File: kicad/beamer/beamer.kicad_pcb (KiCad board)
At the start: 2 copper layers, 117.3 x 83 mm, 65 parts

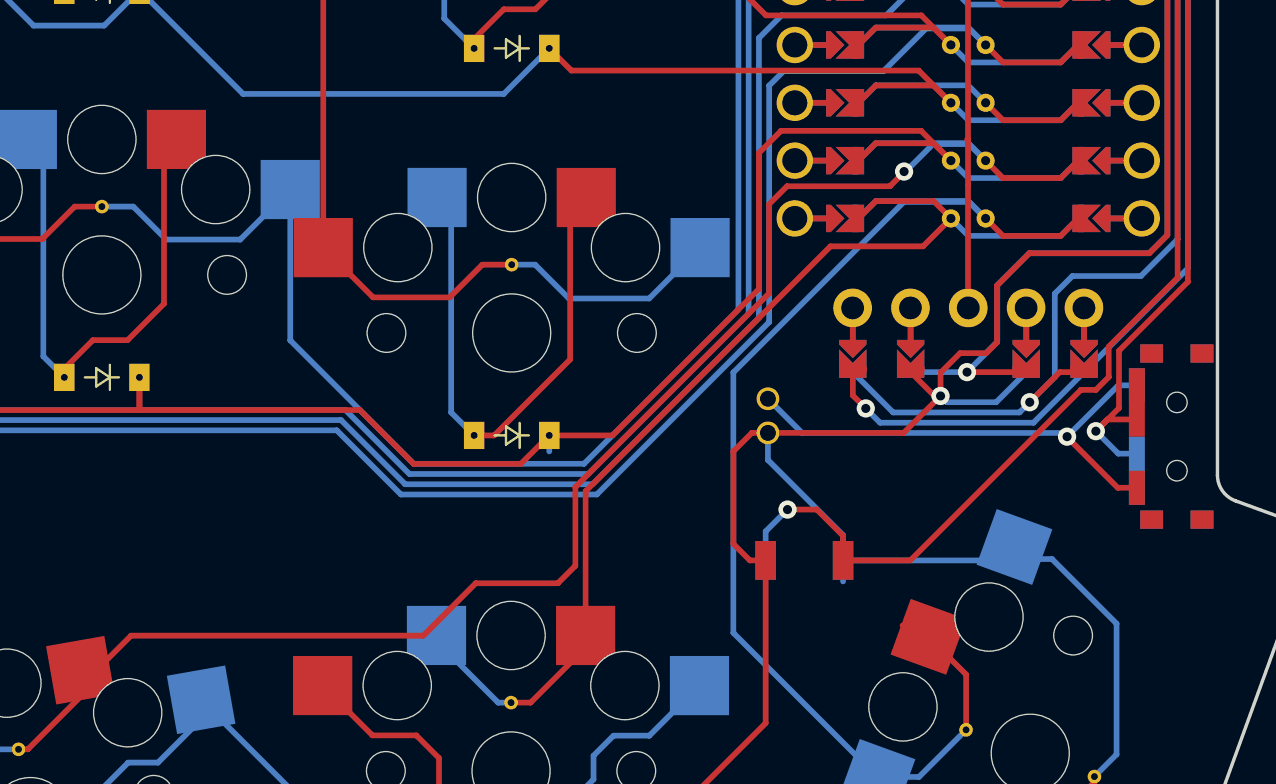
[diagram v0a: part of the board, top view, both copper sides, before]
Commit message: Final changes for printing
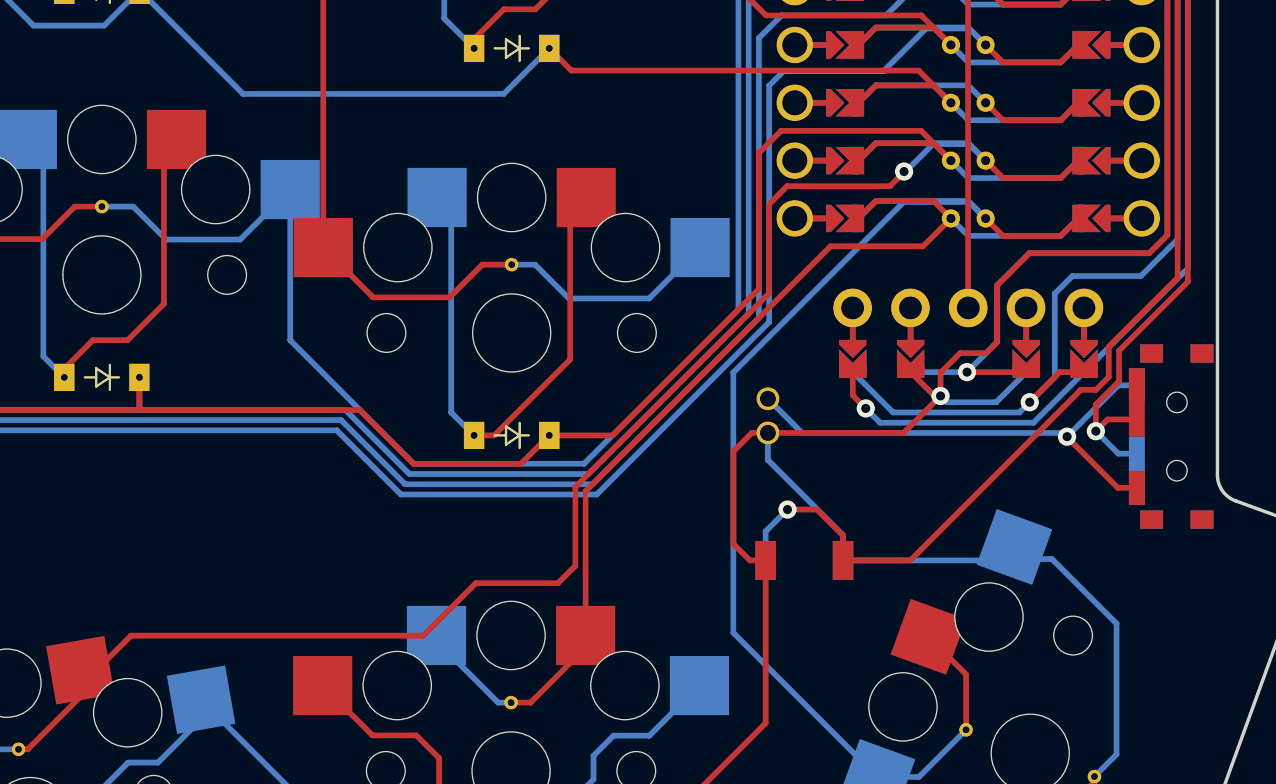
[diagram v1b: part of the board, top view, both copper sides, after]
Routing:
- net P10: track 45.6 -> 44.4 mm
- net GND: track 200.3 -> 199.4 mm
- net P8: track 117.0 -> 116.1 mm
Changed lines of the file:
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@@
       (outputformat 1)
       (mirror false)
-      (drillshape 1)
+      (drillshape 0)
       (scaleselection 1)
-      (outputdirectory "")
+      (outputdirectory "Gerber/")
     )
   )
@@
   (segment (start 158.65 161.2) (end 160.700382 161.2) (width 0.25) (layer "F.Cu") (net 3))
   (segment (start 176.65 149.259378) (end 176.65 148.45) (width 0.25) (layer "F.Cu") (net 3))
-  (segment (start 212.65 148.45) (end 212.65 148.6) (width 0.25) (layer "F.Cu") (net 3))
   (segment (start 222.32912 149.886002) (end 224.693899 152.250781) (width 0.25) (layer "F.Cu") (net 3))
   (segment (start 175.901789 150.007589) (end 176.65 149.259378) (width 0.25) (layer "F.Cu") (net 3))
@@
   (segment (start 239.86 138.594959) (end 240.834601 137.620358) (width 0.25) (layer "F.Cu") (net 3))
   (segment (start 180.054638 148.45) (end 182.292485 146.212153) (width 0.25) (layer "F.Cu") (net 3))
-  (segment (start 230.65 151.704121) (end 230.65 151) (width 0.25) (layer "B.Cu") (net 3))
   (segment (start 159.670356 134.354644) (end 159.670356 140.855062) (width 0.25) (layer "F.Cu") (net 4))
   (segment (start 159.670356 140.855062) (end 157.960229 142.565189) (width 0.25) (layer "F.Cu") (net 4))
@@
   (segment (start 235.045994 164.189093) (end 233.472621 164.189093) (width 0.25) (layer "B.Cu") (net 25))
   (segment (start 243.555 156.49) (end 250.493904 156.49) (width 0.25) (layer "B.Cu") (net 25))
-  (segment (start 243.555 156.49) (end 243.555 157.414572) (width 0.25) (layer "B.Cu") (net 25))
   (segment (start 229.967611 168.737433) (end 228.972654 168.737433) (width 0.25) (layer "B.Cu") (net 25))
   (segment (start 232.594895 165.066819) (end 232.594895 166.110149) (width 0.25) (layer "B.Cu") (net 25))
@@
   (segment (start 251.613064 156.429604) (end 252.731637 156.429604) (width 0.25) (layer "B.Cu") (net 25))
   (segment (start 248.111903 149.541729) (end 250.281271 149.541729) (width 0.25) (layer "B.Cu") (net 25))
-  (segment (start 246.169237 159.345616) (end 246.98806 160.164439) (width 0.25) (layer "F.Cu") (net 26))
   (segment (start 247.306258 159.846241) (end 248.958235 161.498218) (width 0.25) (layer "F.Cu") (net 26))
   (segment (start 248.958235 161.498218) (end 248.958235 163.932694) (width 0.25) (layer "F.Cu") (net 26))
@@
   (segment (start 228.407591 162.737433) (end 228.972654 162.737433) (width 0.25) (layer "B.Cu") (net 27))
   (segment (start 225.697654 159.787433) (end 225.697654 160.027496) (width 0.25) (layer "B.Cu") (net 27))
-  (segment (start 257.254622 114.799263) (end 251.086263 114.799263) (width 0.25) (layer "F.Cu") (net 28))
   (segment (start 254.659212 150.814567) (end 255.173779 150.3) (width 0.25) (layer "F.Cu") (net 28))
-  (segment (start 258.7 116.244641) (end 257.254622 114.799263) (width 0.25) (layer "F.Cu") (net 28))
+  (segment (start 258.7 144.26) (end 258.7 116.244641) (width 0.25) (layer "F.Cu") (net 28))
   (segment (start 255.173779 150.3) (end 256.46 150.3) (width 0.25) (layer "F.Cu") (net 28))
-  (segment (start 256.46 150.3) (end 256.177 150.3) (width 0.25) (layer "F.Cu") (net 28))
-  (segment (start 254.659212 150.814567) (end 255.675947 149.797832) (width 0.25) (layer "F.Cu") (net 28))
-  (segment (start 251.086263 114.799263) (end 249.817 113.53) (width 0.25) (layer "F.Cu") (net 28))
-  (segment (start 255.675947 149.797832) (end 255.675947 147.284053) (width 0.25) (layer "F.Cu") (net 28))
   (segment (start 255.675947 147.284053) (end 258.7 144.26) (width 0.25) (layer "F.Cu") (net 28))
-  (segment (start 258.7 144.26) (end 258.7 116.244641) (width 0.25) (layer "F.Cu") (net 28))
+  (segment (start 257.254622 114.799263) (end 251.086263 114.799263) (width 0.25) (layer "F.Cu") (net 28))
+  (segment (start 254.659212 150.814567) (end 254.659212 149.640184) (width 0.25) (layer "F.Cu") (net 28))
+  (segment (start 254.659212 149.640184) (end 255.675947 148.623449) (width 0.25) (layer "F.Cu") (net 28))
+  (segment (start 251.086263 114.799263) (end 249.817 113.53) (width 0.25) (layer "F.Cu") (net 28))
+  (segment (start 258.7 116.244641) (end 257.254622 114.799263) (width 0.25) (layer "F.Cu") (net 28))
+  (segment (start 255.675947 148.623449) (end 255.675947 147.284053) (width 0.25) (layer "F.Cu") (net 28))
   (via (at 254.659212 150.814567) (size 0.8) (drill 0.4) (layers "F.Cu" "B.Cu") (net 28))
   (segment (start 255.645868 151.8) (end 256.46 151.8) (width 0.25) (layer "B.Cu") (net 28))
@@
   (segment (start 241.114455 154.256464) (end 240.155 155.215919) (width 0.25) (layer "B.Cu") (net 29))
   (segment (start 249.044778 121.922222) (end 249.044778 145.389778) (width 0.25) (layer "F.Cu") (net 30))
-  (segment (start 249.045463 138.045463) (end 249 138) (width 0.25) (layer "F.Cu") (net 30))
   (segment (start 249.817 121.15) (end 249.044778 121.922222) (width 0.25) (layer "F.Cu") (net 30))
-  (segment (start 249.055 140.00126) (end 249.05626 140) (width 0.25) (layer "F.Cu") (net 30))
   (segment (start 249.044778 145.389778) (end 249.045463 145.390463) (width 0.25) (layer "F.Cu") (net 30))
   (segment (start 243.983 149.244598) (end 243.983 148.22) (width 0.25) (layer "F.Cu") (net 32))
